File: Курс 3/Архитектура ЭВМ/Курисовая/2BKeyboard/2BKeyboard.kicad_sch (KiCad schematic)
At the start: 4 parts, among them SW1 SW_Push, SW2 SW_Push, U2 Sparkfun_Pro_Micro

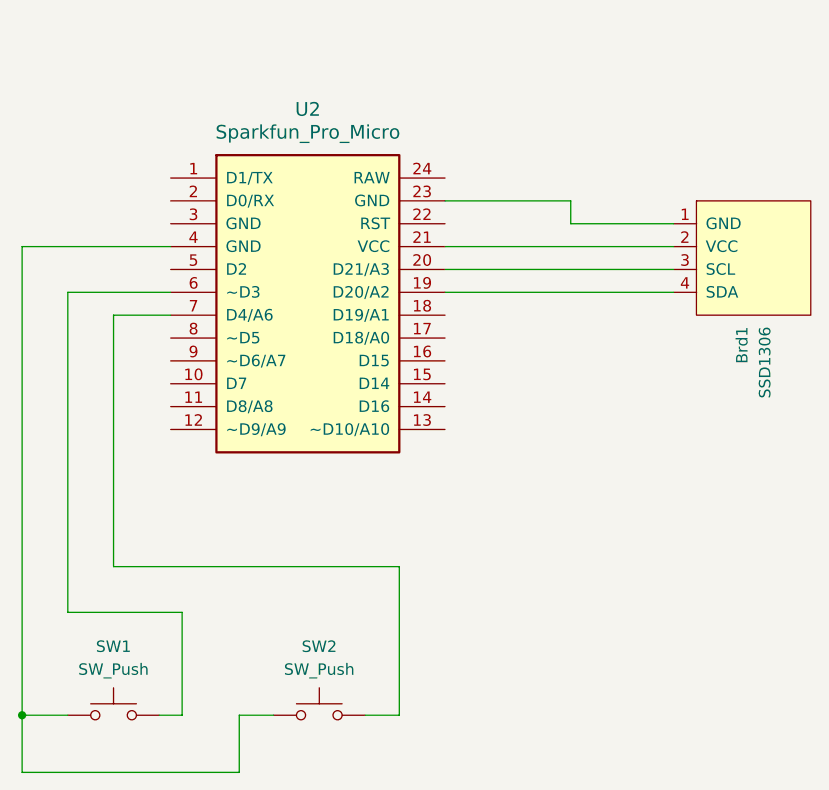
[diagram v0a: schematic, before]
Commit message: vault backup: 2026-03-25 01:54:36
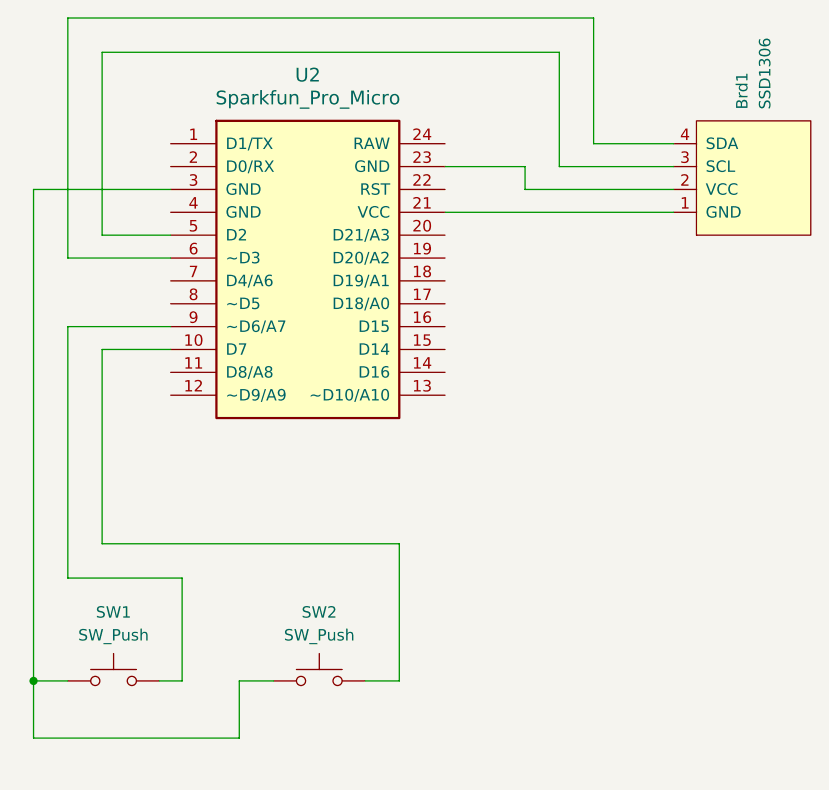
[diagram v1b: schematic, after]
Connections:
- net at Brd1.1 (GND): now also U2.21 (VCC); no longer U2.23 (GND)
- net at Brd1.2 (VCC): now also U2.23 (GND); no longer U2.21 (VCC)
- net at Brd1.3 (SCL): now also U2.5 (D2); no longer U2.20 (D21/A3)
- net at Brd1.4 (SDA): now also U2.6 (~D3); no longer U2.19 (D20/A2)
- net at U2.10 (D7): now also SW2.2
- net at U2.3 (GND): now also SW1.1, SW2.1
- net at SW1.2: now also U2.9 (~D6/A7); no longer U2.6 (~D3)
- net at U2.7 (D4/A6): no longer SW2.2
- now unconnected: U2.4 (GND)
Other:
- moved on the sheet: Brd1, SW1, SW2, U2
